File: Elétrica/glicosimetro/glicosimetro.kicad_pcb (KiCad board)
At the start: 2 copper layers, 96.2 x 67.5 mm, 28 parts, among them Q1 BC337, Q2 BC337, U1 ESP32-C3_SUPERMINI, U3 MCP6002-xMC, U4 LM1117DT-3.3, U6 MCP601R, U7 LTC6910-1CTS8PBF

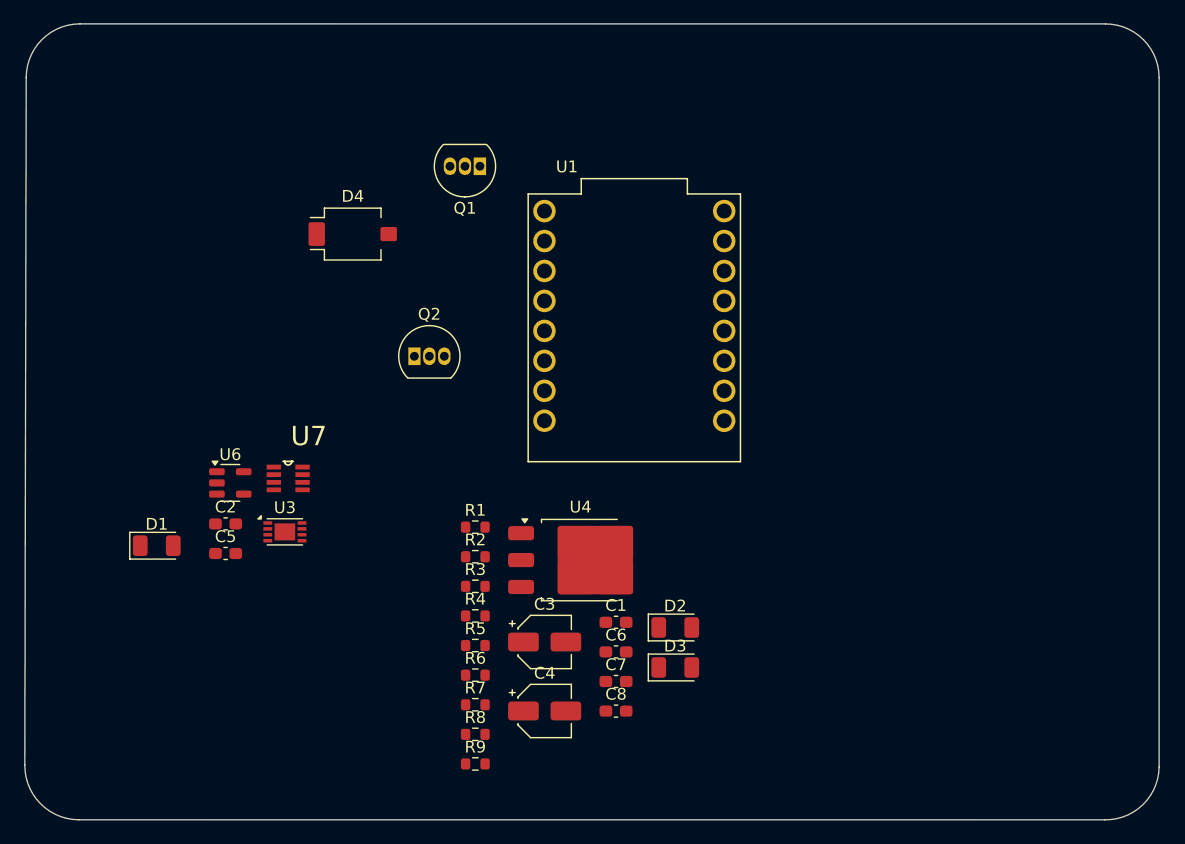
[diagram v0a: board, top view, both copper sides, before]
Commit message: Simulação
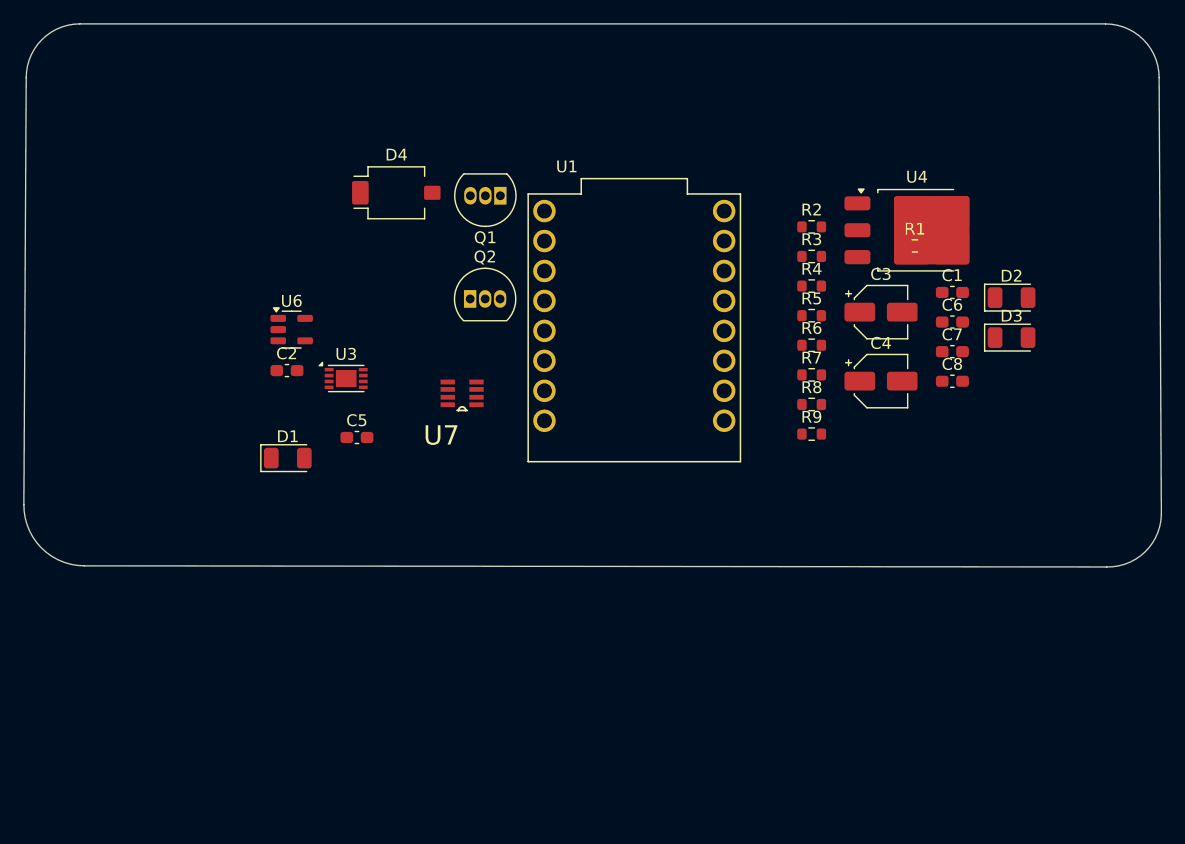
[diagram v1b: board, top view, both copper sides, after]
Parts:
- moved R1 44.3 mm to (206.2, 92.5)
- moved C3 39.9 mm to (203.3, 98.1)
- moved C4 39.9 mm to (203.3, 104.0)
- moved D2 39.9 mm to (214.4, 96.9)
- moved D3 39.9 mm to (214.4, 100.3)
- moved U4 39.9 mm to (206.3, 91.2)
- moved C6 39.9 mm to (209.3, 99.0)
- moved R9 39.9 mm to (197.4, 108.5)
- moved C1 39.9 mm to (209.3, 96.5)
- moved C7 39.9 mm to (209.3, 101.5)
- moved R2 39.9 mm to (197.4, 90.9)
- moved R3 39.9 mm to (197.4, 93.4)
- moved R4 39.9 mm to (197.4, 95.9)
- moved R5 39.9 mm to (197.4, 98.4)
- moved R6 39.9 mm to (197.4, 100.9)
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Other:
- board size 96.2 x 67.5 mm -> 96.5 x 46.1 mm
